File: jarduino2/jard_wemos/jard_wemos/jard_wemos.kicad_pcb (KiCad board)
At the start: 2 copper layers, 52 x 42 mm, 26 parts, among them J1 Conn_01x05, Q1 BPC_2N2222A, Q2 P03P4L-04, U1 BPC_Alim5V, U2 WeMos_D1_mini, U3 24LC01

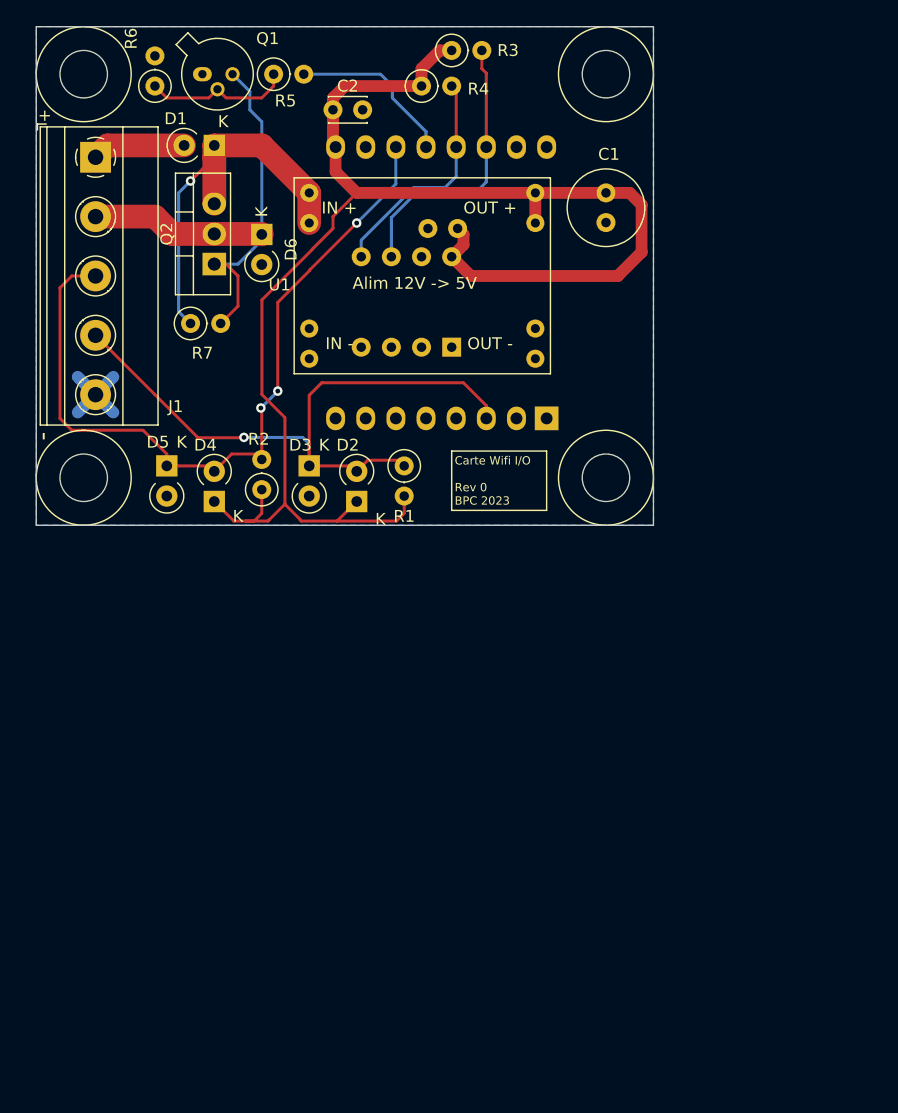
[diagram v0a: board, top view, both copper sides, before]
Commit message: Finalisation carte Wifi I/O
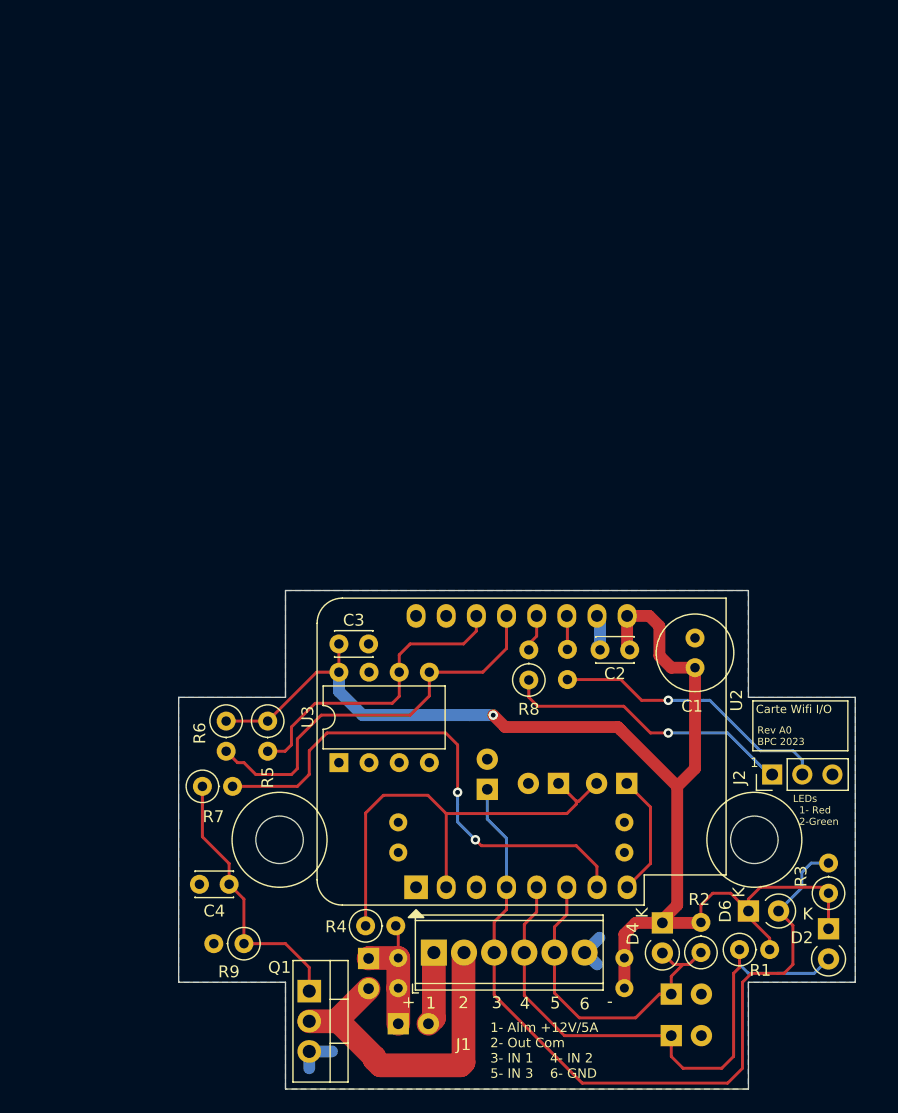
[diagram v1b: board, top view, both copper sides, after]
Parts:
- removed Q2: P03P4L-04, Package_TO_SOT_THT:TO-220-3_Vertical
- removed the REF** at (158.0, 79.0)
- removed the REF** at (114.0, 79.0)
- removed the REF** at (114.0, 45.0)
- removed the REF** at (158.0, 45.0)
- added C4: 100n, Capacitor_THT:C_Disc_D3.0mm_W2.0mm_P2.50mm, F.Cu at (126.2, 113.2)
- added D10: D, Diode_THT:D_A-405_P2.54mm_Vertical_KathodeUp, B.Cu at (138.0, 119.5)
- added D7: D, Diode_THT:D_A-405_P2.54mm_Vertical_KathodeUp, B.Cu at (148.0, 105.2)
- added D8: D, Diode_THT:D_A-405_P2.54mm_Vertical_KathodeUp, B.Cu at (159.8, 104.8)
- added D9: D, Diode_THT:D_A-405_P2.54mm_Vertical_KathodeUp, B.Cu at (154.0, 104.8)
- added J2: LEDs, Connector_PinHeader_2.54mm:PinHeader_1x03_P2.54mm_Vertical, F.Cu at (172.0, 104.0)
- added R10: 100, Resistor_THT:R_Axial_DIN0207_L6.3mm_D2.5mm_P2.54mm_Vertical, B.Cu at (154.8, 96.0)
- added R8: 100, Resistor_THT:R_Axial_DIN0207_L6.3mm_D2.5mm_P2.54mm_Vertical, F.Cu at (151.5, 96.0)
- added R9: 100k, Resistor_THT:R_Axial_DIN0207_L6.3mm_D2.5mm_P2.54mm_Vertical, F.Cu at (127.5, 118.2)
- added REF**: BPC_Trou4mm_Fixation, bpc:BPC_Trou4mm_Fixation, F.Cu at (170.5, 109.5)
- added REF**: BPC_Trou4mm_Fixation, bpc:BPC_Trou4mm_Fixation, F.Cu at (130.5, 109.5)
- C3, U2, U3: moved to F.Cu
- D1, D3, D5, U1: moved to B.Cu
- J1: footprint TerminalBlock_Phoenix:TerminalBlock_Phoenix_MKDS-1,5-5_1x05_P5.00mm_Horizontal -> TerminalBlock_Phoenix:TerminalBlock_Phoenix_MPT-0,5-6-2.54_1x06_P2.54mm_Horizontal
- Q1: value BPC_2N2222A -> BPC_IPP034N03L; footprint Package_TO_SOT_THT:TO-18-3 -> Package_TO_SOT_THT:TO-220-3_Vertical
- R3: value 10k -> 100k
- R4: value 10k -> 1,2M
- R5: value 50 -> 10k
- R6: value 100k -> 10k
- R7: value 100k -> 50
- moved R3 77.8 mm to (176.8, 114.0), turned to 90 degrees
- moved Q1 77.8 mm to (133.0, 122.2), turned to 270 degrees
- moved D1 75.6 mm to (140.5, 125.0), turned to 0 degrees
- moved J1 72.8 mm to (143.5, 119.0), turned to 0 degrees
- moved R4 70.9 mm to (137.8, 116.8)
- moved D6 70.2 mm to (170.0, 115.5), turned to 0 degrees
- moved U1 67.4 mm to (140.5, 122.0)
- moved D5 61.5 mm to (163.5, 122.5), turned to 0 degrees
- moved D3 56.9 mm to (163.5, 126.0), turned to 0 degrees
- moved R5 54.5 mm to (129.5, 99.5), turned to 270 degrees
- moved R6 53.8 mm to (126.0, 99.5), turned to 270 degrees
- moved R2 53.8 mm to (166.0, 119.0)
- moved D2 53.6 mm to (176.8, 117.0), turned to 270 degrees
- moved C2 51.9 mm to (160.0, 93.5), turned to 180 degrees
- moved D4 51.8 mm to (162.8, 116.5), turned to 270 degrees
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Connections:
- D4 pad 2: IN_1 -> IN_3
- D5 pad 1: IN_1 -> IN_3
- D6 pad 1: OUT_12V -> +5V
- D6 pad 2: GND -> IN_1
- J1 pad 2: OUT_12V -> OUT_12V_COM
- J1 pad 5: GND -> IN_3
- Q1 pad 1: GND -> Net-(C4-Pad1)
- Q1 pad 2: Net-(Q1-Pad2) -> OUT_12V_COM
- Q1 pad 3: Net-(Q1-Pad3) -> GND
- R2 pad 1: +5V -> IN_3
- R2 pad 2: IN_1 -> +5V
- R3 pad 2: Net-(R3-Pad2) -> IN_1
- R4 pad 1: +5V -> POW_MES
- R4 pad 2: Net-(R4-Pad2) -> +12V
- R5 pad 1: Net-(Q1-Pad2) -> +5V
- R5 pad 2: CMD_OUT_12V -> Net-(R5-Pad2)
- R6 pad 1: Net-(Q1-Pad2) -> +5V
- R6 pad 2: GND -> Net-(R6-Pad2)
- R7 pad 1: +12V -> Net-(C4-Pad1)
- R7 pad 2: Net-(Q1-Pad3) -> CMD_OUT_12V
- U2 pad 11: IN_1 -> LED_VERTE
- U2 pad 12: CMD_OUT_12V -> LED_ROUGE
- U2 pad 13: Net-(R4-Pad2) -> Net-(R6-Pad2)
- U2 pad 14: Net-(R3-Pad2) -> Net-(R5-Pad2)
- U2 pad 2: Net-(U2-Pad2) -> POW_MES
- U2 pad 3: IN_2 -> Net-(U2-Pad3)
- U2 pad 4: Net-(U2-Pad4) -> IN_1
- U2 pad 5: Net-(U2-Pad5) -> IN_2
- U2 pad 6: Net-(U2-Pad6) -> IN_3
- U2 pad 7: Net-(U2-Pad7) -> CMD_OUT_12V
- U3 pad 5: Net-(R4-Pad2) -> Net-(R6-Pad2)
- U3 pad 6: Net-(R3-Pad2) -> Net-(R5-Pad2)
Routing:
- net POW_MES: track 0.00 -> 39.7 mm
- net Net-(R6-Pad2): track 0.00 -> 34.2 mm
- net CMD_OUT_12V: track 14.2 -> 44.0 mm, vias 0 -> 2
- net IN_3: track 0.00 -> 27.9 mm
- net OUT_12V_COM: track 0.00 -> 27.8 mm
- net Net-(Q1-Pad3): track 26.9 -> 0.00 mm
- net Net-(R5-Pad2): track 0.00 -> 26.0 mm
- net Net-(J2-Pad1): track 0.00 -> 24.7 mm, vias 0 -> 1
- net Net-(J2-Pad2): track 0.00 -> 23.8 mm, vias 0 -> 1
- net Net-(R3-Pad2): track 23.8 -> 0.00 mm
- net Net-(C4-Pad1): track 0.00 -> 23.3 mm
- net +12V: track 32.8 -> 10.9 mm, vias 1 -> 0
- net Net-(R4-Pad2): track 19.4 -> 0.00 mm
- net OUT_12V: track 14.6 -> 0.00 mm
- net Net-(Q1-Pad2): track 12.4 -> 0.00 mm
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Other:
- board size 52 x 42 mm -> 57 x 42 mm
- board text added: "1- Alim +12V/5A 2- Out Com 3- IN 1 4- IN 2 5- IN 3 6- GND"
- board text added: "6"
- board text added: "Carte Wifi I/O"
- board text added: "LEDs 1- Red 2-Green"
- board text added: "Rev A0 BPC 2023"
- board text removed: "+12V"
- board text removed: "CMD"
- board text removed: "Carte Wifi I/O Rev 0 BPC 2023"
- board text removed: "GND"
- board text removed: "IN 1"
- board text removed: "IN 2"
